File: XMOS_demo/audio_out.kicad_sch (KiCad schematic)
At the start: 26 parts, among them J3 AudioJack3_SwitchT, U5 MAX97220C

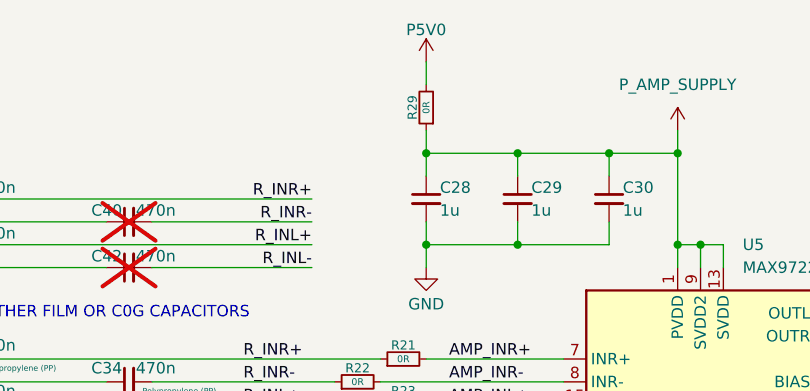
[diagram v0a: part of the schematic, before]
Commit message: sch work, pcb import and initial board outline
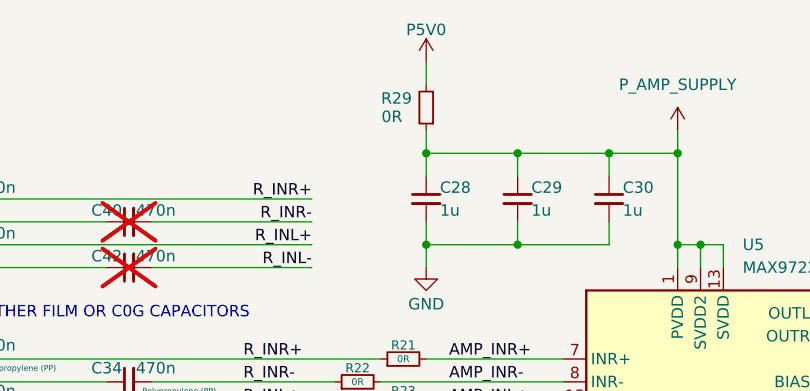
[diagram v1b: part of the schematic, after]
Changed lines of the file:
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@@
 		(dnp no)
 		(property "Reference" "R29"
-			(at 115.316 58.42 90)
+			(at 113.538 57.404 0)
 			(effects
 				(font
-					(size 1.016 1.016)
+					(size 1.27 1.27)
 				)
 			)
 		)
 		(property "Value" "0R"
-			(at 116.84 58.42 90)
+			(at 113.03 59.436 0)
 			(effects
 				(font
-					(size 0.762 0.762)
+					(size 1.27 1.27)
 				)
 			)
